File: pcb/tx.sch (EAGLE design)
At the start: 9 parts

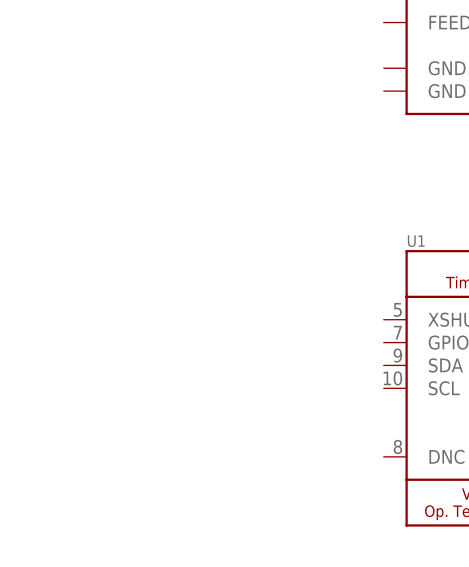
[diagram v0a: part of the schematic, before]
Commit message: dt rx done
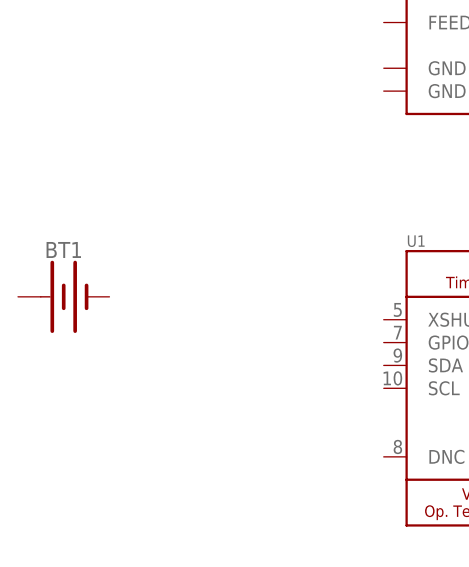
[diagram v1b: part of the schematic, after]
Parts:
- added BT1: (no value), SparkFun-Batteries:BATTERY-24.5MM_PTH
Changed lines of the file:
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@@
 <?xml version="1.0" encoding="utf-8"?>
 <!DOCTYPE eagle SYSTEM "eagle.dtd">
-<eagle version="9.1.0">
+<eagle version="9.1.3">
 <drawing>
 <settings>
-<setting alwaysvectorfont="no"/>
+<setting alwaysvectorfont="yes"/>
 <setting verticaltext="up"/>
 </settings>
@@
 <part name="U$7" library="L1" deviceset="M3_MOUNTING_HOLE" device=""/>
 <part name="U$8" library="L1" deviceset="M3_MOUNTING_HOLE" device=""/>
+<part name="BT1" library="SparkFun-Batteries" deviceset="BATTERY" device="-24.5MM_PTH"/>
 </parts>
 <sheets>
@@
 <instance part="U$7" gate="G$1" x="-30.48" y="-17.78"/>
 <instance part="U$8" gate="G$1" x="-45.72" y="-20.32"/>
+<instance part="BT1" gate="G$1" x="-53.34" y="43.18"/>
 </instances>
 <busses>

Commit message: before tx firmware test
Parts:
- added C1, C3: 100nF, clock:CAP0805
- added C10: 4.7µF, SparkFun-Passives:CAP0805
- added C11, C12: 4.7uF, clock:CAP0805
- added C2, C6: 2.2nF, clock:CAP0805
- added C4: 1.5pF, clock:CAP0805
- added C5: 1pF, clock:CAP0805
- added C7: 4.7pF, clock:CAP0805
- added C8, C9: 22pF, clock:CAP0805
- added D1, D2: BAT20J, SparkFun-DiscreteSemi:DIODE-SCHOTTKY-BAT20J
- added L1: 3.9nH, basicBoard:INDUCTOR0805
- added L2: 8.2nH, basicBoard:INDUCTOR0805
- added L3: 2.7nH, basicBoard:INDUCTOR0805
- added LED1: (no value), joyAnalog:LEDCHIP-LED0805
- added R1: 22K, joyAnalog:RESISTOR0805-RES
- added R2, R3: 5K1, joyAnalog:RESISTOR0805-RES
- added R4: 4.7K, SparkFun-Passives:RESISTOR0805-RES
- added R5: 27K, SparkFun-Passives:RESISTOR0805-RES
- added S2: (no value), Adafruit Feather M0 Adalogger:SWITCH-SPDT-SMD-A
- added U$9: XC6206_DEV, 3pos_slide_switch:XC6206_DEV
- added U3: MCP73831T-2ACI/OT, microbuilder:MCP73831/2
- added Y1: CRYSTAL-26MHZSMD-3.2X2.5, SparkFun-Clocks:CRYSTAL-26MHZSMD-3.2X2.5
- BT1: device SparkFun-Batteries:BATTERY-24.5MM_PTH -> tx:TX_SPARKFUN-BATTERIES_BATTERY-24.5MM_PTH
- U$1: value USBC_6P_DEV -> L1_USBC_6P_DEV; device L1:USBC_6P_DEV -> tx:L1_USBC_6P_DEV
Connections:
- new net +3V3: C1.1, C12.1, C2.1, U$3.VDD@15, U$3.VDD@18, U$3.VDD@7, U$9.OUT
- new net GND: BT1.+, C1.2, C10.2, C11.2, C12.2, C2.2, C3.2, C5.2, C6.2, C7.2, C8.2, C9.2, R1.2, R2.2, R3.2, R5.2, U$1.GND, U$3.VSS@0, U$3.VSS@14, U$3.VSS@17, U$3.VSS@20, U$3.VSS@8, U$9.GND, U3.VSS, Y1.3
- new net N$1: C3.1, U$3.DVDD
- new net N$10: R3.1, U$1.CC2
- new net N$11: R2.1, U$1.CC1
- new net N$12: LED1.C, R4.1
- new net N$13: R4.2, U3.STAT
- new net N$14: U$3.MOSI
- new net N$15: U$3.MISO
- new net N$16: U$3.SCK
- new net N$17: R5.1, U3.PROG
- new net N$19: D2.A, S2.P
- new net N$2: R1.1, U$3.IREF
- new net N$20: U$3.CSN
- new net N$21: U$3.CE
- new net N$25: BT1.-, C10.1, S2.S, U3.VBAT
- new net N$26: D1.A, U$1.VBUS
- new net N$27: C11.1, D1.C, D2.C, LED1.A, U$9.IN, U3.VDD
- new net N$3: L1.1, L2.1, U$3.ANT2
- new net N$4: C4.1, L1.2
- new net N$5: C4.2, C5.1
- new net N$6: L2.2, L3.1, U$3.ANT1
- new net N$7: C8.1, U$3.XC2, Y1.1
- new net N$8: C6.1, C7.1, L3.2, U$3.VDD_PA
- new net N$9: C9.1, U$3.XC1, Y1.2
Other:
- note added: "Charge current: I_CHG = 1000 / R_PROG"
- moved on the sheet: BT1, U$3
